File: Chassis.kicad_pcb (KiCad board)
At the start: 2 copper layers, 120 x 120 mm, 31 parts, among them IC1 RT6285GSP, J1 FR_JST, J10 BL_XT30, J11 Sabre Vertical Header 6, J2 FR_XT30, J3 BR_JST, J4 BR_XT30, J5 IN_JST, J6 IN_XT60, J7 FL_JST, J8 FL_XT30, J9 BL_JST

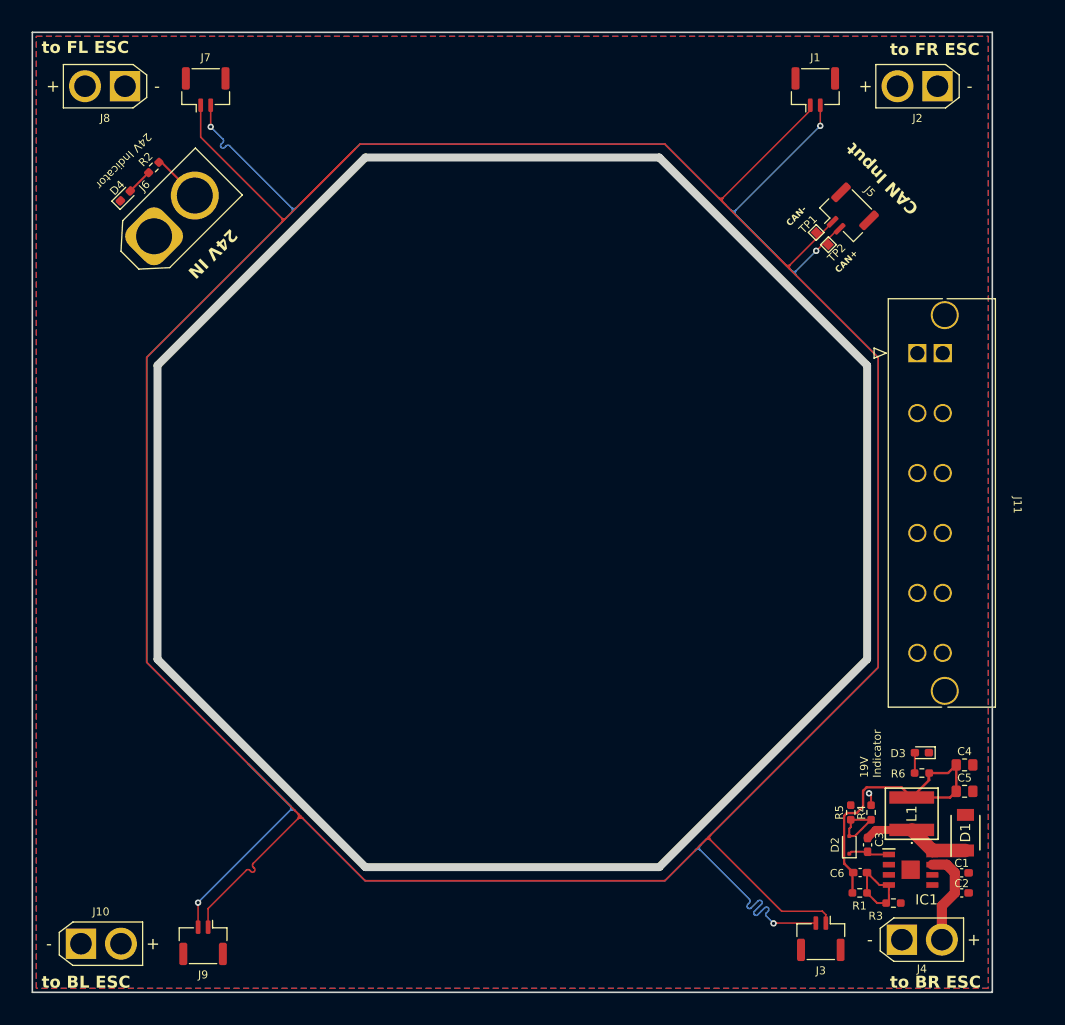
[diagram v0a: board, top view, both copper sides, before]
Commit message: Add power connector
big boy
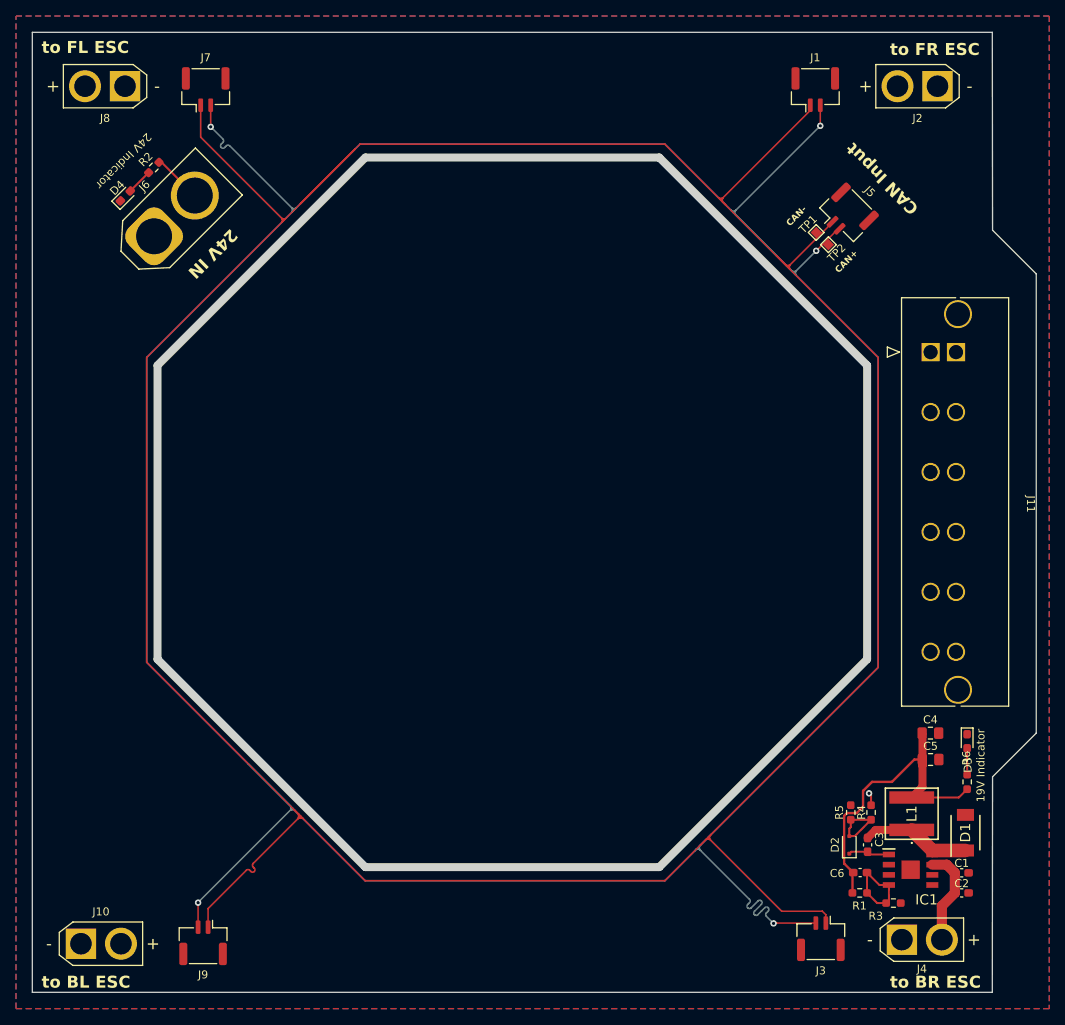
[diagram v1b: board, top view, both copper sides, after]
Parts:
- moved D3 5.84 mm to (205.2, 118.9), turned to -90 degrees
- moved C4 5.83 mm to (200.6, 117.9)
- moved C5 5.82 mm to (200.7, 121.2)
- moved R6 5.77 mm to (205.2, 124.0), turned to 90 degrees
- moved J11 1.66 mm to (203.8, 70.2)
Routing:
- net /V_{OUT}: track 38.7 -> 40.7 mm
- net Net-(D3-A): track 2.56 -> 3.29 mm
- removed copper zone on F.Cu, net /V_{OUT}
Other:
- board size 120 x 120 mm -> 125.5 x 120 mm
